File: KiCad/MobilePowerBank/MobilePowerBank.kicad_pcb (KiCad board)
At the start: 2 copper layers, 138 x 195 mm, 217 parts, among them J1 Power IN, J10 Power OUT 6, J2 Power OUT 2, J3 Power OUT 1, J4 OLED I2C, J5 PDI, J6 OLED, J7 Power OUT 3, J8 Power OUT 4, J9 Power OUT 5, SW1 SW_DIP_x01, U1 INA169, U10 INA138, U11 LMZ14201H, U12 LMZ14201H, U13 INA138, U14 INA138, U15 ATXMEGA256A3U-AU, U16 INA138, U2 LMZ14203H, U3 L78M12, U4 INA138, U5 UA78M33, U6 LMZ14203H, U7 LMZ14203H, U8 LMZ14203H, U9 INA138, x1 jumper, x2 jumper, x3 jumper, x4 jumper, x5 jumper

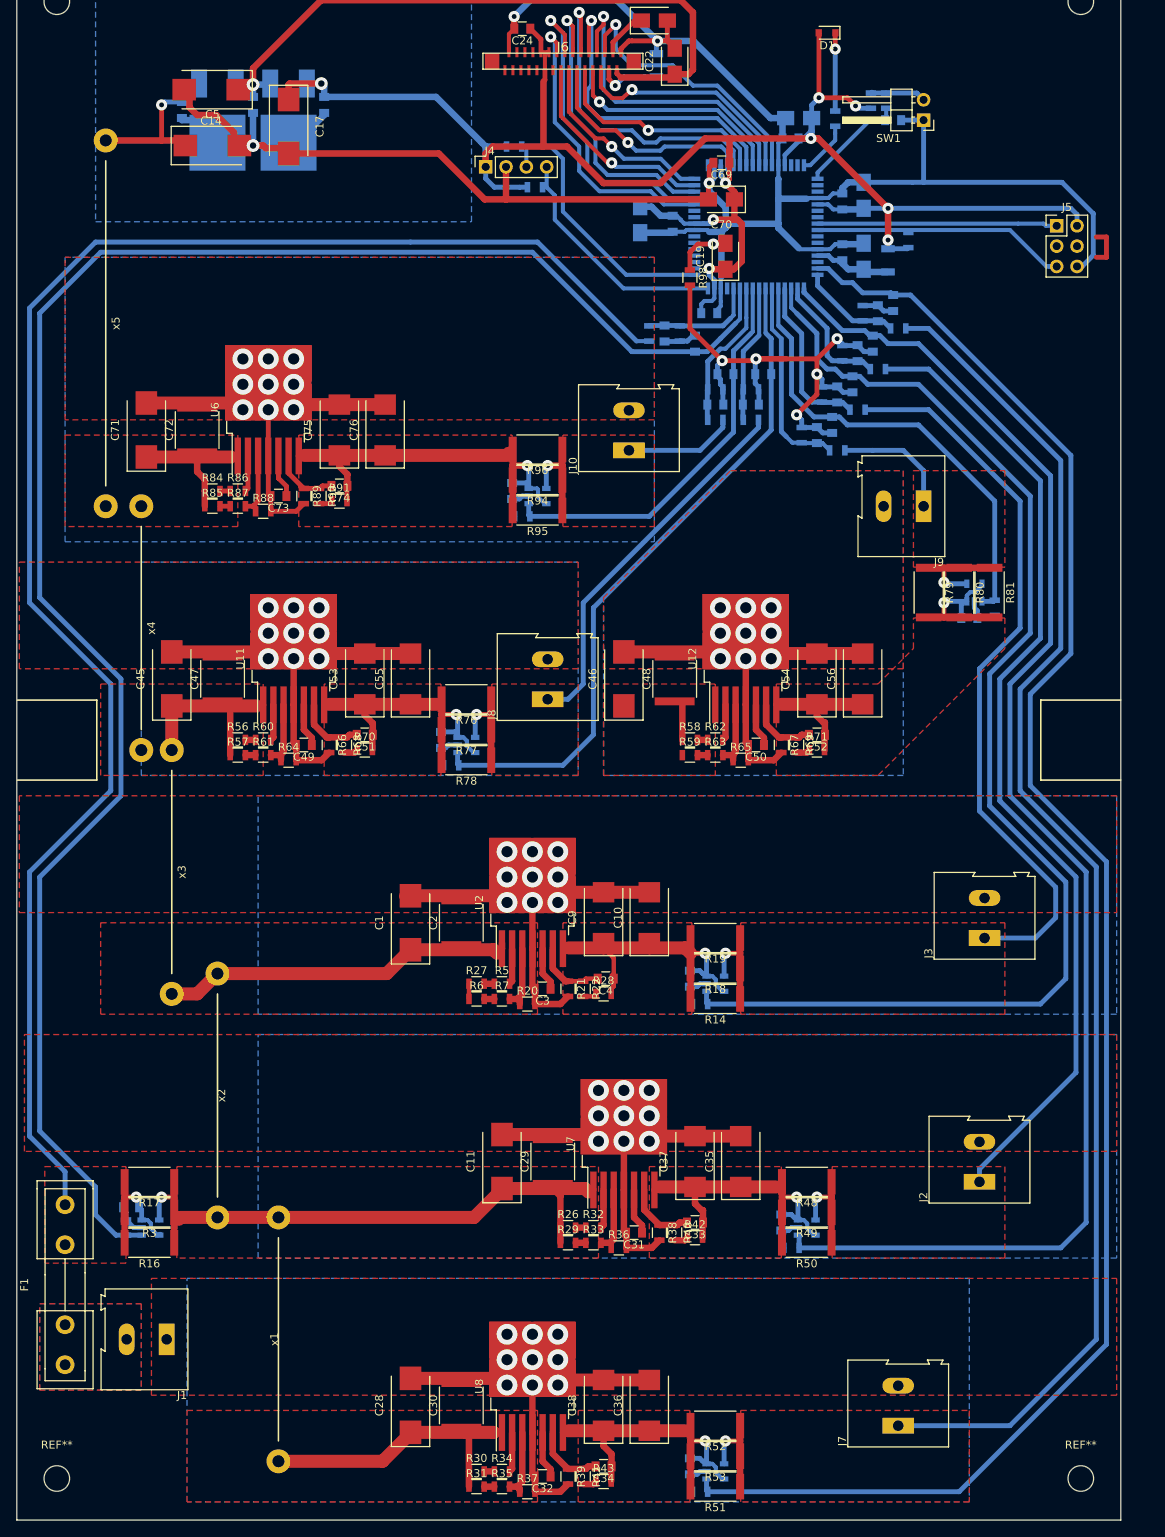
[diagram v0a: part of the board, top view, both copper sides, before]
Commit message: PCB finish, BOM check
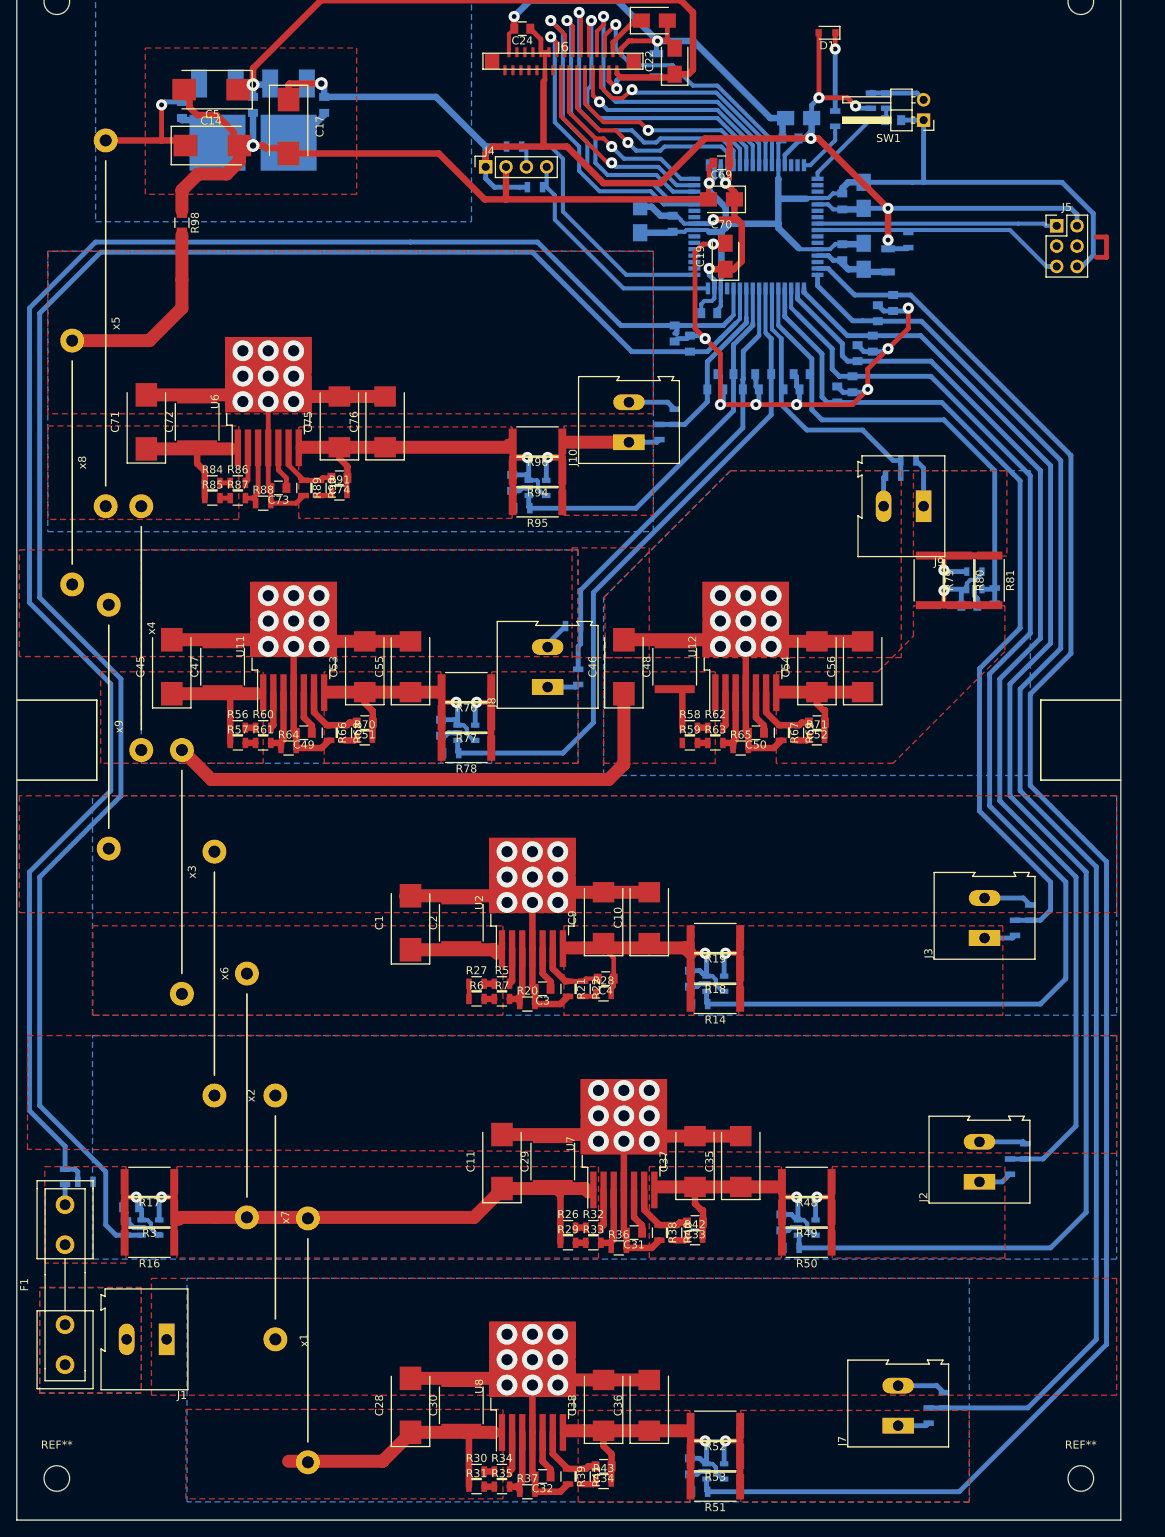
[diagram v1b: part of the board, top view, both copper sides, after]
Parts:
- added x6: jumper, JPJumpers:Jumper_30x1.5, F.Cu at (44.7, 146.7)
- added x7: jumper, JPJumpers:Jumper_30x1.5, F.Cu at (52.3, 177.2)
- added x8: jumper, JPJumpers:Jumper_30x1.5, F.Cu at (26.9, 82.8)
- added x9: jumper, JPJumpers:Jumper_30x1.5, F.Cu at (31.5, 115.8)
- moved R47 136.3 mm to (135.9, 200.0)
- moved R46 135.9 mm to (134.0, 201.9), turned to 90 degrees
- moved R2 129.5 mm to (28.6, 172.7), turned to 0 degrees
- moved R1 128.2 mm to (26.0, 172.1)
- moved R45 102.4 mm to (146.1, 168.9)
- moved R44 101.1 mm to (144.1, 170.8), turned to 90 degrees
- moved R13 69.8 mm to (146.7, 139.1)
- moved R12 67.7 mm to (144.8, 141.0), turned to 90 degrees
- moved R98 63.9 mm to (40.6, 52.8)
- moved R72 38.7 mm to (90.2, 109.6), turned to 90 degrees
- moved R73 37.0 mm to (89.5, 103.3), turned to 180 degrees
- moved R75 12.5 mm to (129.5, 84.5), turned to 180 degrees
- moved R74 8.98 mm to (131.4, 82.5)
- moved C62 7.41 mm to (118.1, 71.8), turned to 180 degrees
- moved R92 7.15 mm to (100.3, 79.0), turned to 90 degrees
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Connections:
- C26 pad 2: GNDA -> GND
- C27 pad 2: GNDA -> GND
- C39 pad 2: GNDA -> GND
- C43 pad 2: GNDA -> GND
- C46 pad 1: POWER_IN -> POWER_IN_4
- C48 pad 1: POWER_IN -> POWER_IN_4
- C57 pad 2: GNDA -> GND
- C58 pad 2: GNDA -> GND
- C61 pad 2: GNDA -> GND
- C62 pad 2: GNDA -> GND
- C7 pad 1: GND -> GNDA
- C77 pad 2: GNDA -> GND
- C79 pad 2: GNDA -> GND
- R2 pad 2: GND -> GNDA
- R4 pad 2: GND -> GNDA
- R58 pad 1: POWER_IN -> POWER_IN_4
- R59 pad 1: POWER_IN -> POWER_IN_4
- U1 pad 2: GND -> GNDA
- U12 pad 1: POWER_IN -> POWER_IN_4
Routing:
- net IN_Voltage: track 14.5 -> 220.5 mm
- net VDD: track 224.1 -> 18.3 mm
- net OUT_3_Voltage: track 12.7 -> 181.2 mm
- net POWER_3_OUT: track 183.7 -> 16.3 mm
- net OUT_2_Voltage: track 16.0 -> 139.4 mm
- net POWER_2_OUT: track 136.2 -> 16.6 mm
- net OUT_1_Voltage: track 20.8 -> 109.0 mm
- net POWER_1_OUT: track 104.5 -> 16.3 mm
- net GND: track 306.8 -> 391.0 mm, vias 5 -> 12
- net POWER_IN_4: track 24.1 -> 89.5 mm
- net POWER_4_OUT: track 59.7 -> 16.3 mm
- net OUT_4_Voltage: track 17.3 -> 57.0 mm
- net POWER_IN_1: track 46.6 -> 14.4 mm
- net GNDA: track 436.9 -> 424.9 mm, vias 59 -> 54
- net OUT_5_Voltage: track 25.4 -> 34.7 mm
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- added copper zone on F.Cu, net GND
